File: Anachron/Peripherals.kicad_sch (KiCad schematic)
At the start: 21 parts, among them J3 Motor Pads, SW2 Pad, U4 BMI270, U5 MAX98357A

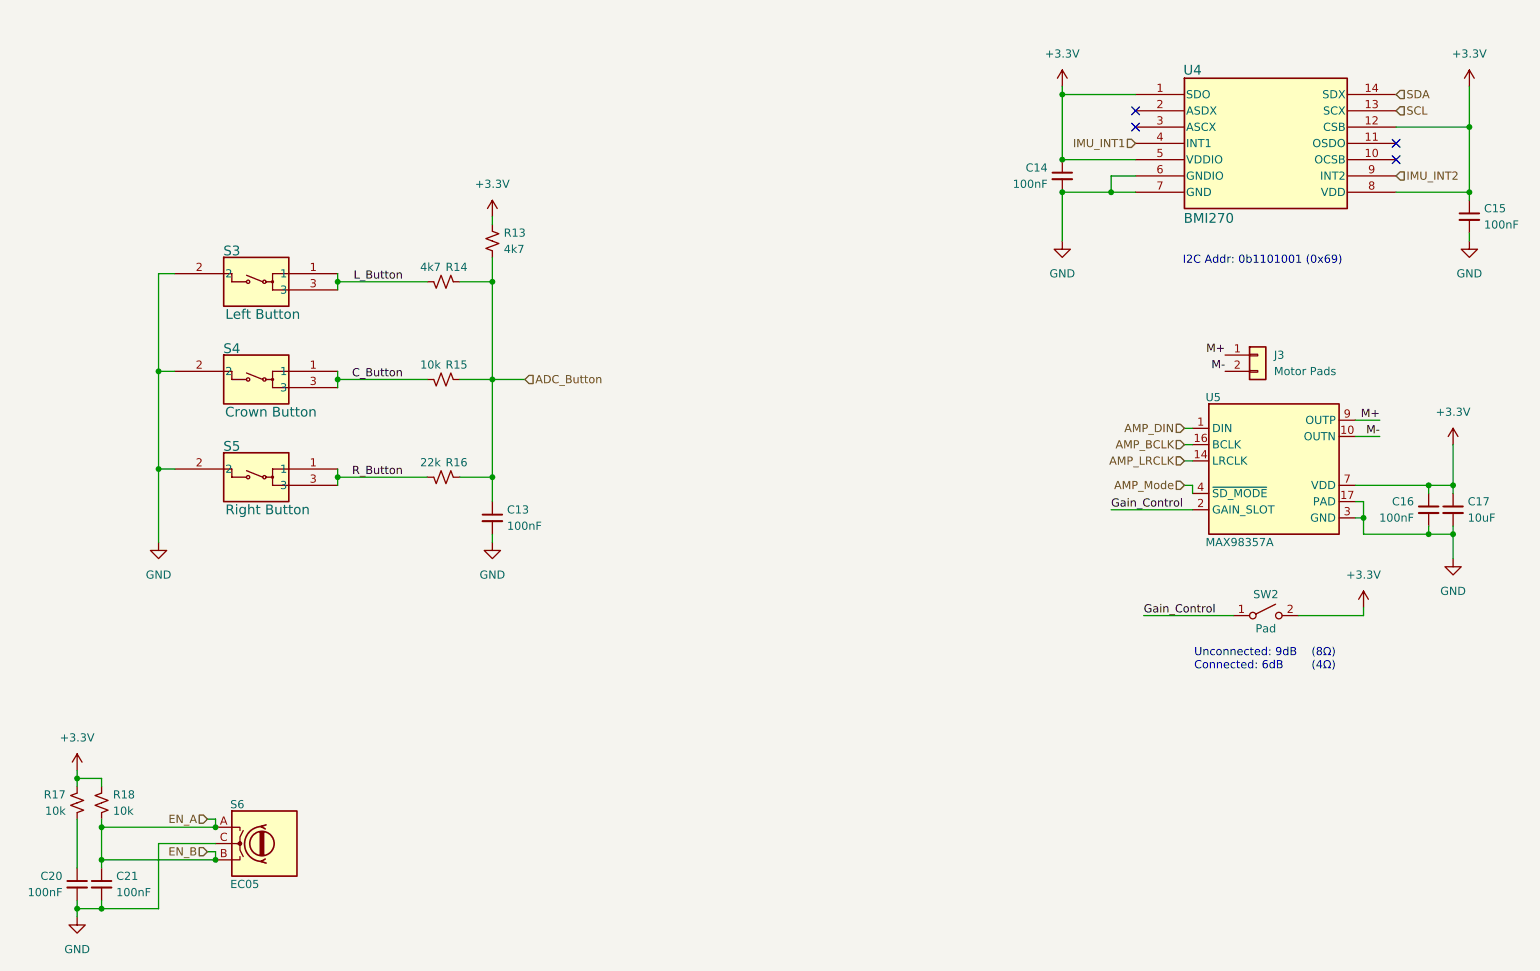
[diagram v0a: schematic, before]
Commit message: layout power
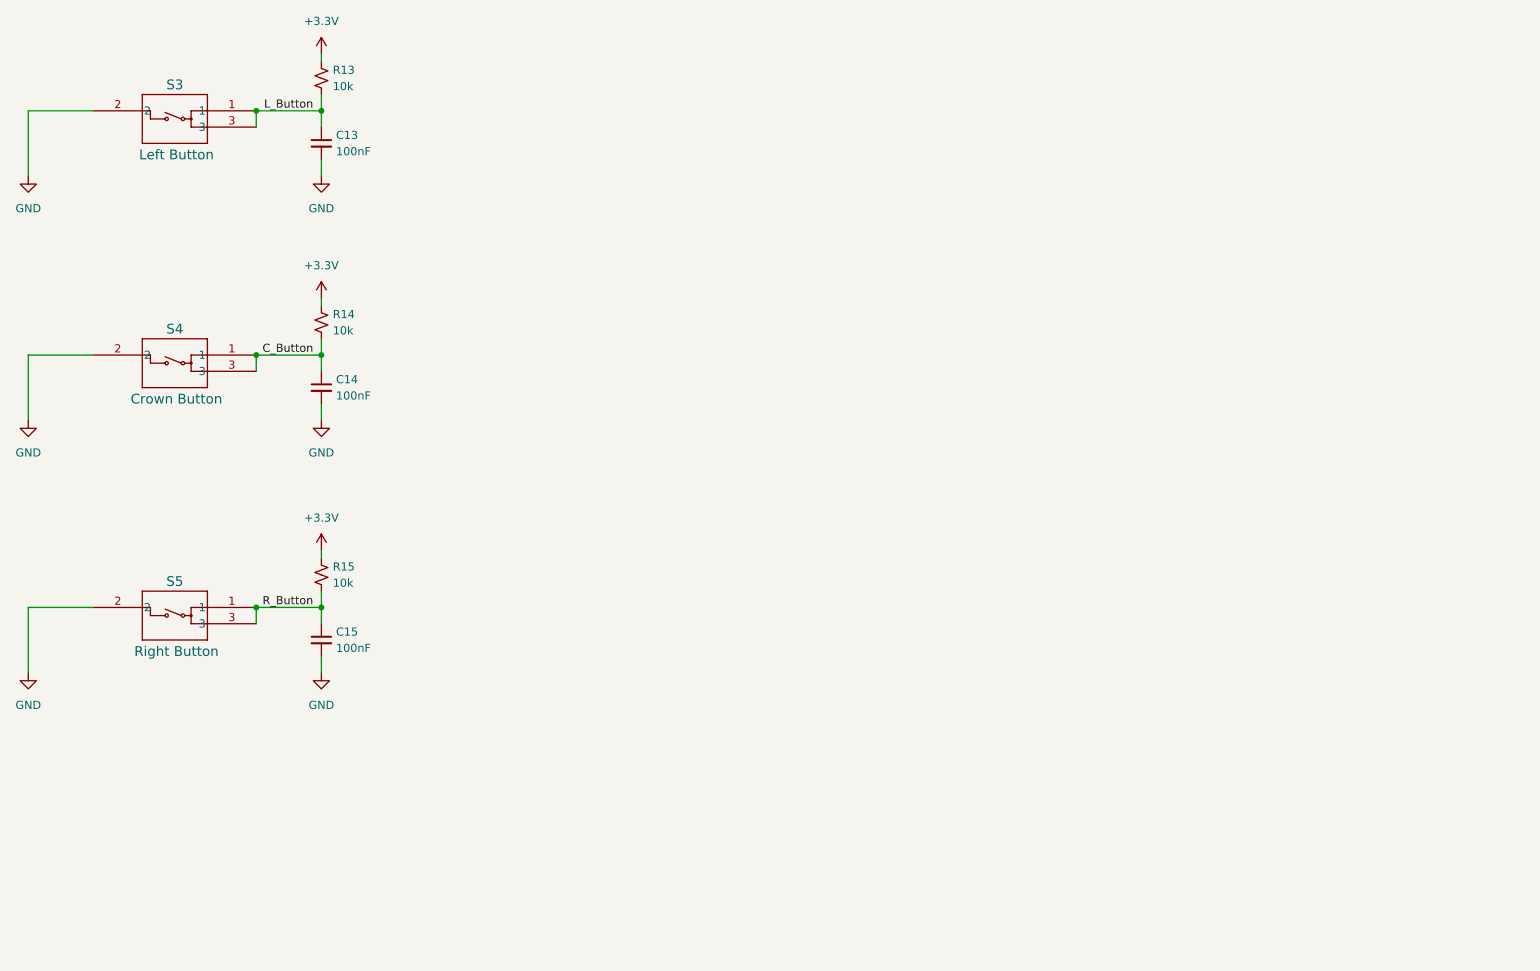
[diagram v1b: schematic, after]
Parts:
- removed C16, C20, C21: 100nF, Capacitor_SMD:C_0603_1608Metric, symbol Device:C_Small
- removed C17: 10uF, Capacitor_SMD:C_0805_2012Metric, symbol Device:C_Small
- removed J3: Motor Pads, symbol Connector_Generic:Conn_01x02
- removed R16: 22k, Resistor_SMD:R_0603_1608Metric, symbol Device:R_Small_US
- removed R17, R18: 10k, Resistor_SMD:R_0603_1608Metric, symbol Device:R_Small_US
- removed S6: EC05, footprints:EC05 Encoder, symbol Device:RotaryEncoder
- removed SW2: Pad, Jumper:SolderJumper-2_P1.3mm_Open_RoundedPad1.0x1.5mm, symbol Switch:SW_SPST
- removed U4: BMI270, footprints:BMI270_BOS-M, symbol symbols:BMI270
- removed U5: MAX98357A, Package_DFN_QFN:TQFN-16-1EP_3x3mm_P0.5mm_EP1.23x1.23mm_ThermalVias, symbol Audio:MAX98357A
- R13, R14: value 4k7 -> 10k
- S3, S4, S5: footprint PTS845_CNK -> footprints:PTS845_CNK
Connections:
- net +3.3V: now also R14.1, R15.1; no longer C14.1, C15.1
- net C_Button: now also C14.1, R14.2; no longer R15.1
- net L_Button: now also C13.1, R13.2; no longer R14.1
- net R_Button: now also C15.1, R15.2
- removed net ADC_Button: C13.1, R13.2, R14.2, R15.2
- no-connect marks 4 -> 0
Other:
- note removed: "(8Ω) (4Ω)"
- note removed: "I2C Addr: 0b1101001 (0x69)"
- note removed: "Unconnected: 9dB Connected: 6dB"
- moved on the sheet: C13, R13

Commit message: layed everything outttt
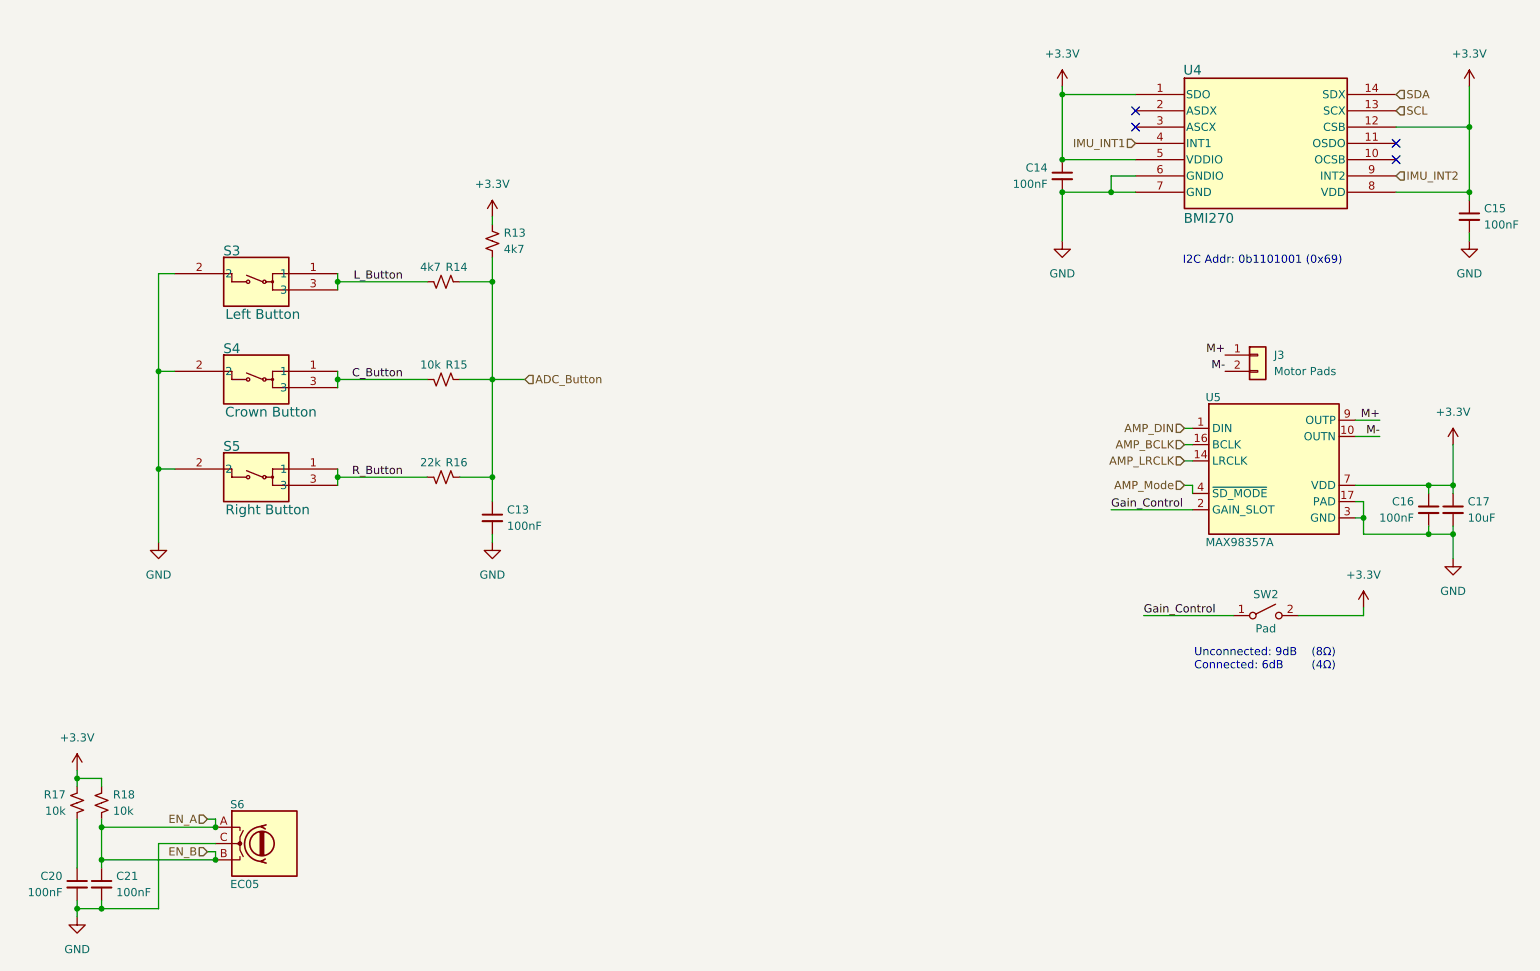
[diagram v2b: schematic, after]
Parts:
- added C16, C20, C21: 100nF, Capacitor_SMD:C_0603_1608Metric, symbol Device:C_Small
- added C17: 10uF, Capacitor_SMD:C_0805_2012Metric, symbol Device:C_Small
- added J3: Motor Pads, symbol Connector_Generic:Conn_01x02
- added R16: 22k, Resistor_SMD:R_0603_1608Metric, symbol Device:R_Small_US
- added R17, R18: 10k, Resistor_SMD:R_0603_1608Metric, symbol Device:R_Small_US
- added S6: EC05, footprints:EC05 Encoder, symbol Device:RotaryEncoder
- added SW2: Pad, Jumper:SolderJumper-2_P1.3mm_Open_RoundedPad1.0x1.5mm, symbol Switch:SW_SPST
- added U4: BMI270, footprints:BMI270_BOS-M, symbol symbols:BMI270
- added U5: MAX98357A, Package_DFN_QFN:TQFN-16-1EP_3x3mm_P0.5mm_EP1.23x1.23mm_ThermalVias, symbol Audio:MAX98357A
- R13, R14: value 10k -> 4k7
- S3, S4, S5: footprint footprints:PTS845_CNK -> PTS845_CNK
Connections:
- net +3.3V: now also C14.1, C15.1, C16.1, C17.1, R17.1, R18.1, SW2.2 (B), U4.1 (SDO), U4.12 (CSB), U4.5 (VDDIO), U4.8 (VDD), U5.7 (VDD); no longer R14.1, R15.1
- net C_Button: now also R15.1; no longer C14.1, R14.2
- net GND: now also C16.2, C17.2, C20.2, C21.2, S6.C, U4.6 (GNDIO), U4.7 (GND), U5.17 (PAD), U5.3 (GND)
- net L_Button: now also R14.1; no longer C13.1, R13.2
- net R_Button: now also R16.1; no longer C15.1, R15.2
- new net: C20.1, R17.2
- new net: U5.11 (GND), U5.15 (GND)
- new net ADC_Button: C13.1, R13.2, R14.2, R15.2, R16.2
- new net AMP_BCLK: U5.16 (BCLK)
- new net AMP_DIN: U5.1 (DIN)
- new net AMP_LRCLK: U5.14 (LRCLK)
- new net AMP_Mode: U5.4 (~{SD_MODE})
- new net EN_A: C21.1, R18.2, S6.A, S6.B
- new net Gain_Control: SW2.1 (A), U5.2 (GAIN_SLOT)
- new net IMU_INT1: U4.4 (INT1)
- new net IMU_INT2: U4.9 (INT2)
- new net M+: J3.1 (Pin_1), U5.9 (OUTP)
- new net M-: J3.2 (Pin_2), U5.10 (OUTN)
- new net SCL: U4.13 (SCX)
- new net SDA: U4.14 (SDX)
- no-connect marks 0 -> 4
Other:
- note added: "(8Ω) (4Ω)"
- note added: "I2C Addr: 0b1101001 (0x69)"
- note added: "Unconnected: 9dB Connected: 6dB"
- moved on the sheet: C13, R13
